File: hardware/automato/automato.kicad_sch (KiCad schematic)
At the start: 59 parts, among them J1 Motor1, J2 Motor2, J3 Motor4, J4 Motor3, J5 Servo 1, J6 i2c, J7 Servo 2, J8 Relay 1, J9 Relay 2, K1 G5Q-1A, K2 G5Q-1A, Q1 AO3400A, Q2 AO3400A, Q3 AO3400A, Q4 AO3400A, Q5 AO3400A, Q6 AO3400A, U1 ESP32-C6-DEVKITC-1-N8, U3 AP63357DV-7

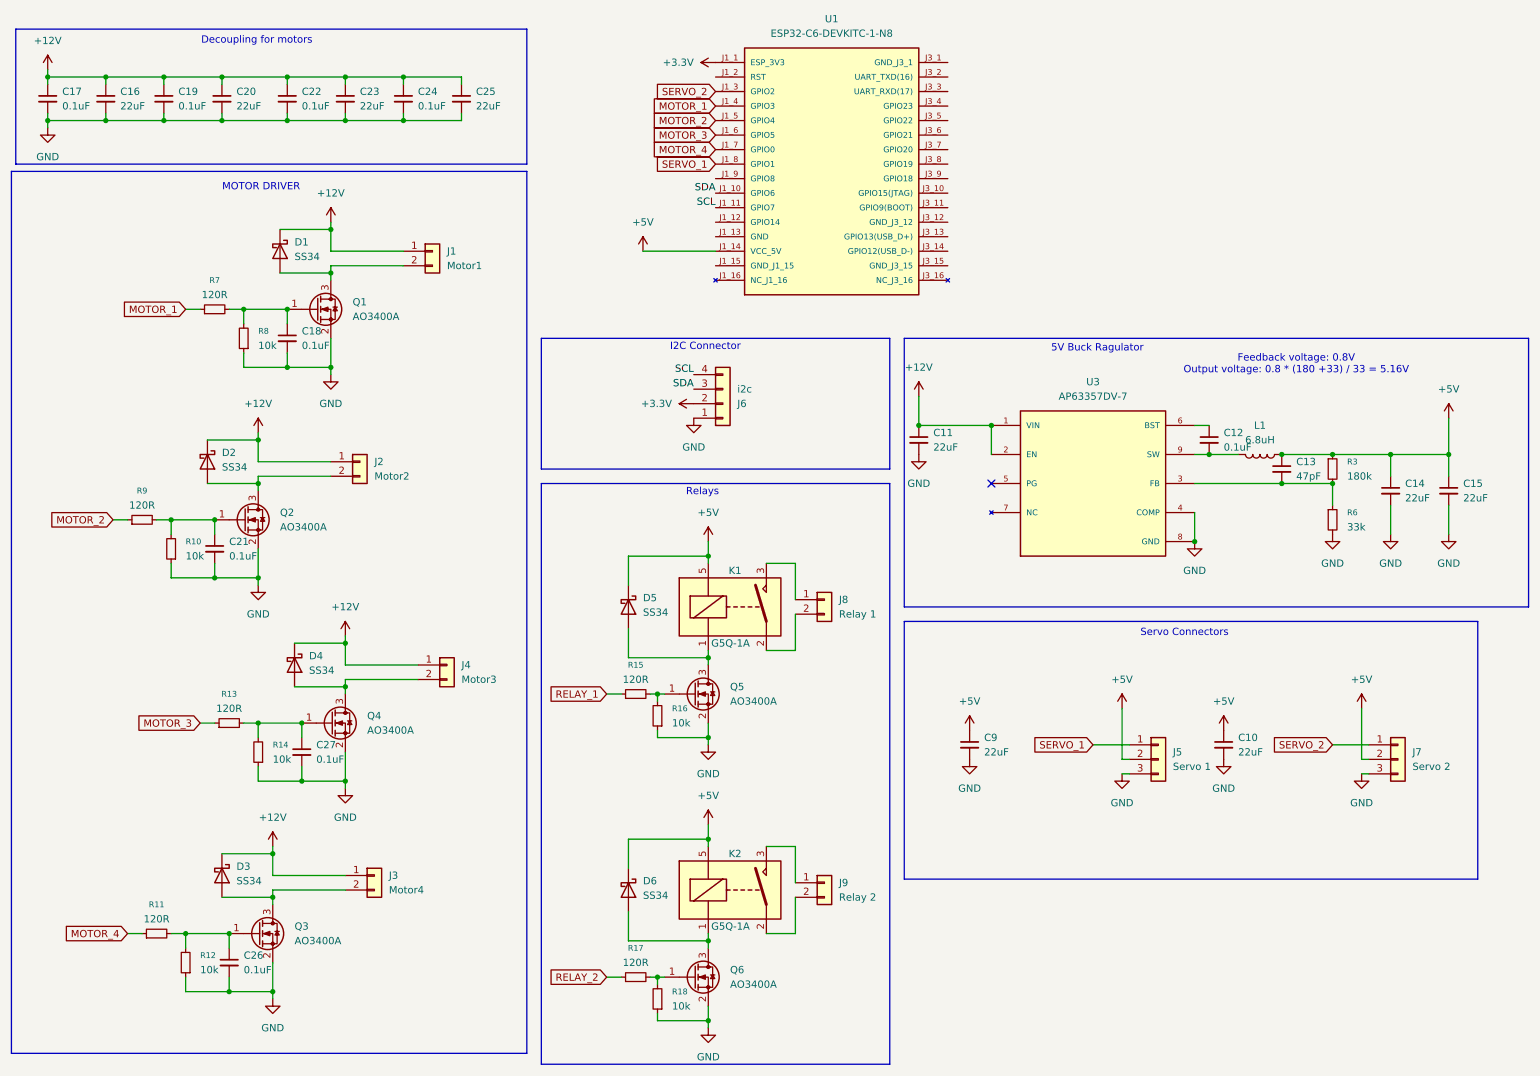
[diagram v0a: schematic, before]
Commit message: started layout
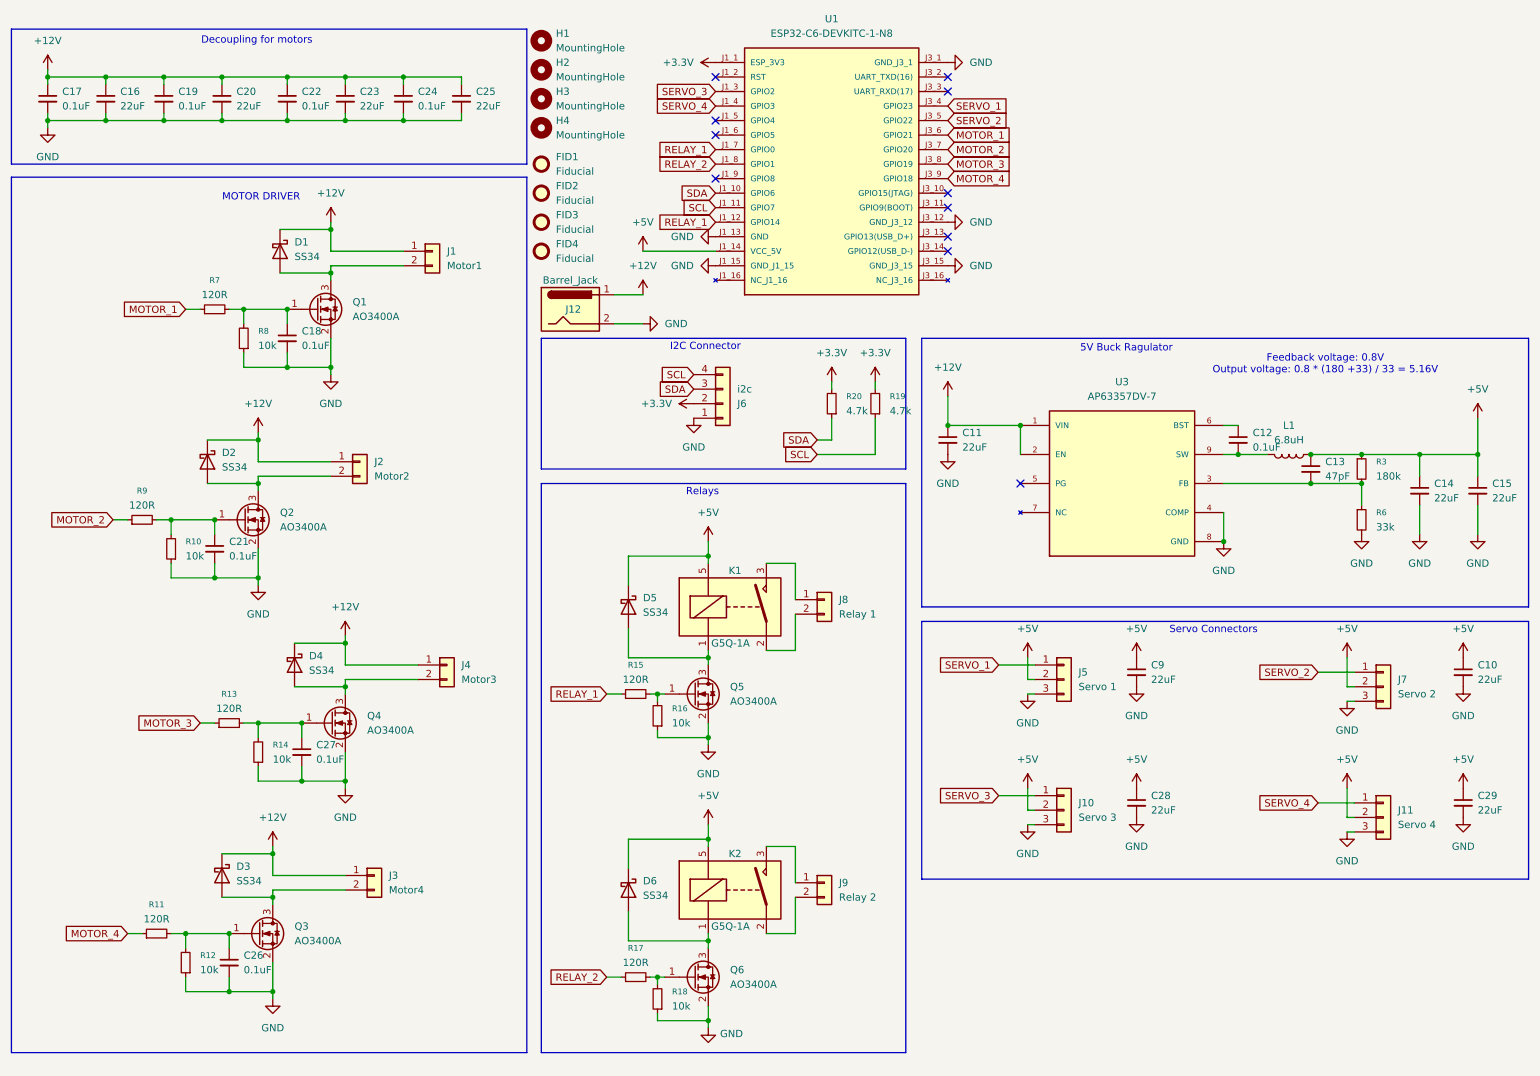
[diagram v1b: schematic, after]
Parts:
- added C28, C29: 22uF, Capacitor_SMD:C_0805_2012Metric, symbol Device:C_Small
- added FID1, FID2, FID3, FID4: Fiducial, Fiducial:Fiducial_1.5mm_Mask3mm, symbol Mechanical:Fiducial
- added H1, H2, H3, H4: MountingHole, MountingHole:MountingHole_3.2mm_M3, symbol Mechanical:MountingHole
- added J10: Servo 3, Connector_PinHeader_2.54mm:PinHeader_1x03_P2.54mm_Vertical, symbol Connector_Generic:Conn_01x03
- added J11: Servo 4, Connector_PinHeader_2.54mm:PinHeader_1x03_P2.54mm_Vertical, symbol Connector_Generic:Conn_01x03
- added J12: Barrel_Jack, Connector_BarrelJack:BarrelJack_Horizontal, symbol Connector:Barrel_Jack
- added R19, R20: 4.7k, Resistor_SMD:R_0603_1608Metric, symbol Device:R_Small
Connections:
- net +12V: now also J12.1
- net +3.3V: now also R19.2, R20.2
- net +5V: now also C28.1, C29.1, J10.2 (Pin_2), J11.2 (Pin_2)
- net GND: now also U1.J1_13 (GND), U1.J1_15 (GND_J1_15), U1.J3_1 (GND_J3_1), U1.J3_12 (GND_J3_12), U1.J3_15 (GND_J3_15), C28.2, C29.2, J10.3 (Pin_3), J11.3 (Pin_3), J12.2
- net MOTOR_1: now also U1.J3_6 (GPIO21); no longer U1.J1_4 (GPIO3)
- net MOTOR_2: now also U1.J3_7 (GPIO20); no longer U1.J1_5 (GPIO4)
- net MOTOR_3: now also U1.J3_8 (GPIO19); no longer U1.J1_6 (GPIO5)
- net MOTOR_4: now also U1.J3_9 (GPIO18); no longer U1.J1_7 (GPIO0)
- net RELAY_1: now also U1.J1_12 (GPIO14), U1.J1_7 (GPIO0)
- net RELAY_2: now also U1.J1_8 (GPIO1)
- net SCL: now also R19.1
- net SDA: now also R20.1
- net SERVO_1: now also U1.J3_4 (GPIO23); no longer U1.J1_8 (GPIO1)
- net SERVO_2: now also U1.J3_5 (GPIO22); no longer U1.J1_3 (GPIO2)
- new net SERVO_3: J10.1 (Pin_1), U1.J1_3 (GPIO2)
- new net SERVO_4: J11.1 (Pin_1), U1.J1_4 (GPIO3)
- no-connect marks 1 -> 11
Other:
- moved on the sheet: C10, C11, C12, C13, C14, C15, C9, J5, J7, L1, R3, R6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
